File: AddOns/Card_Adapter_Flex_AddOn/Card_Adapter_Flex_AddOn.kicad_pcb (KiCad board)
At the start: 4 copper layers, 57.4 x 27 mm, 28 parts, among them J1 17-pin-FPC, J2 4-pin-FPC, U1 5PB1214CMGK8, U3 5PB1214CMGK8

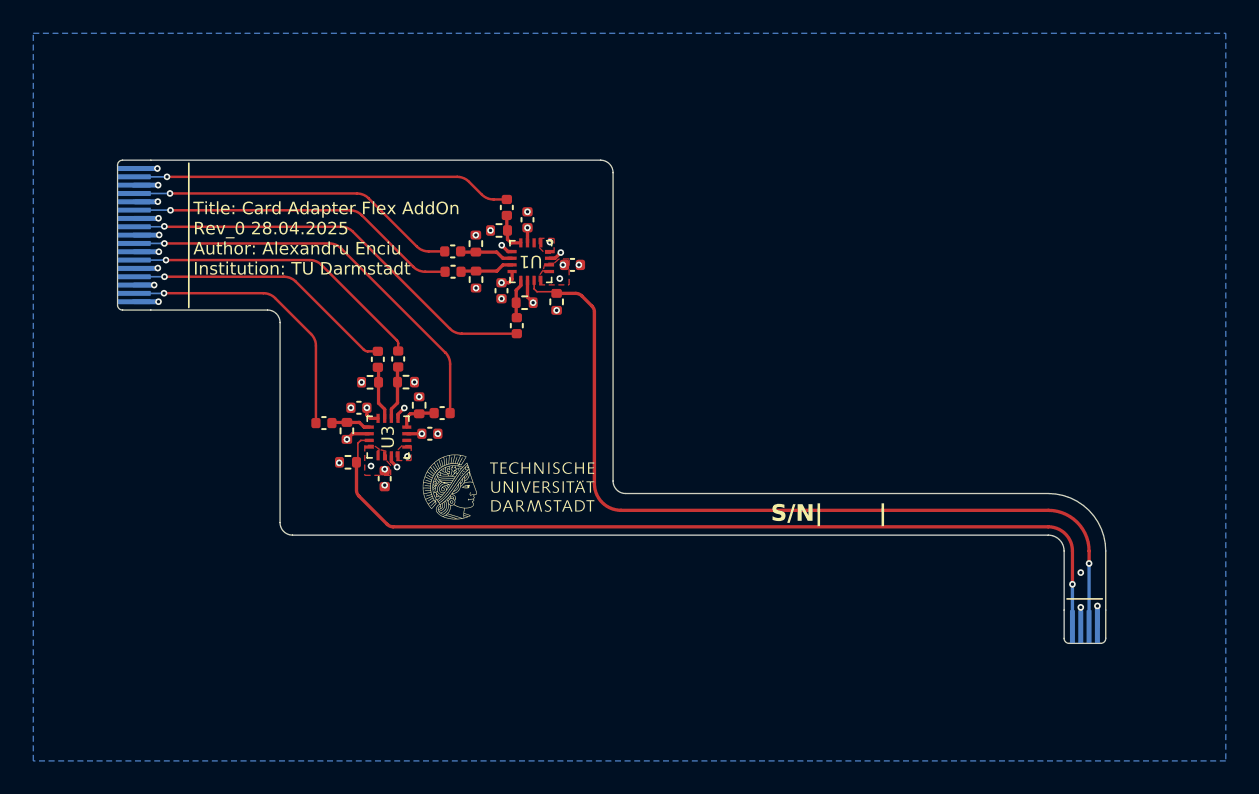
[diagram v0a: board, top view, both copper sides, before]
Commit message: .
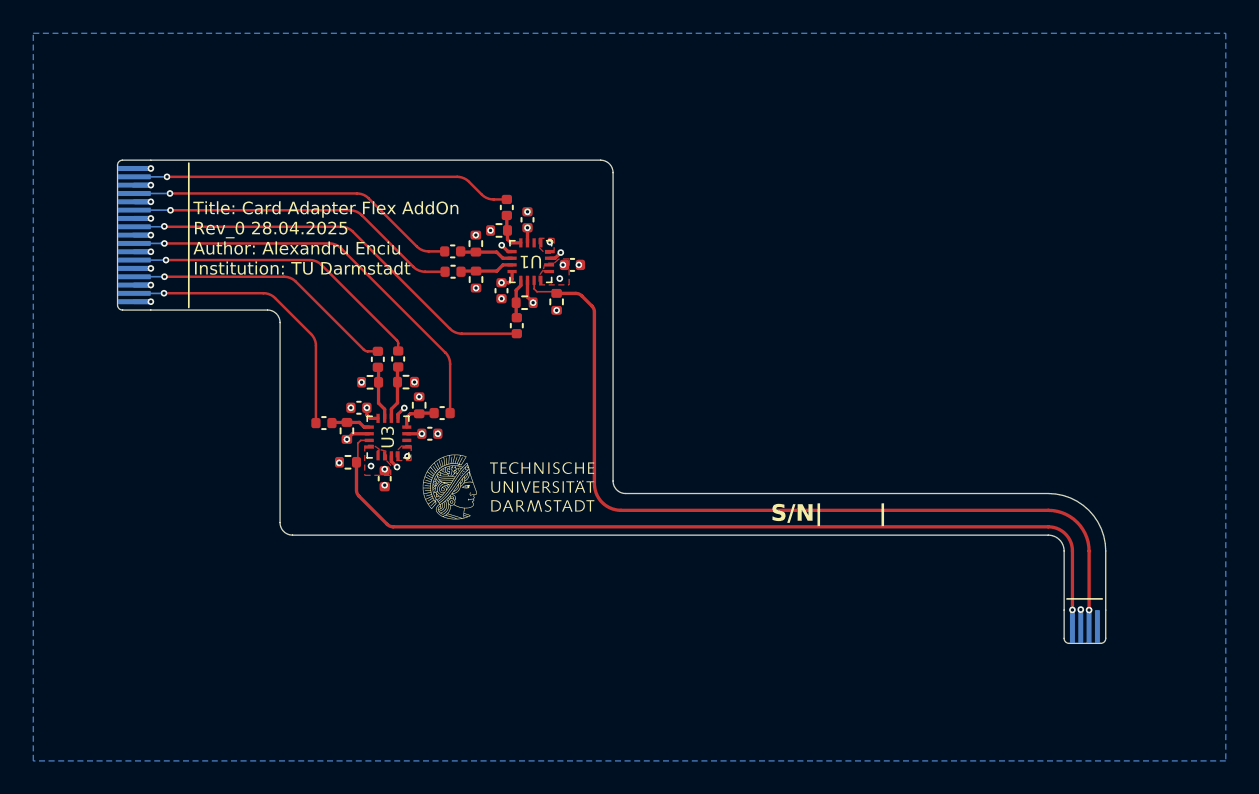
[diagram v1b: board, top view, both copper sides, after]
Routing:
- net GND: track 20.1 -> 16.2 mm, vias 31 -> 30
- net +3V3: track 5.44 -> 4.19 mm, vias 11 -> 10
- added copper zone on In1.Cu, net GND
